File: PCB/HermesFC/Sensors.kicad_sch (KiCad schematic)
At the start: 16 parts, among them U4 MPU-6050, U5 BMP280, U6 LD39015M18R, U7 NTS0104PW, U8 ICM-20948

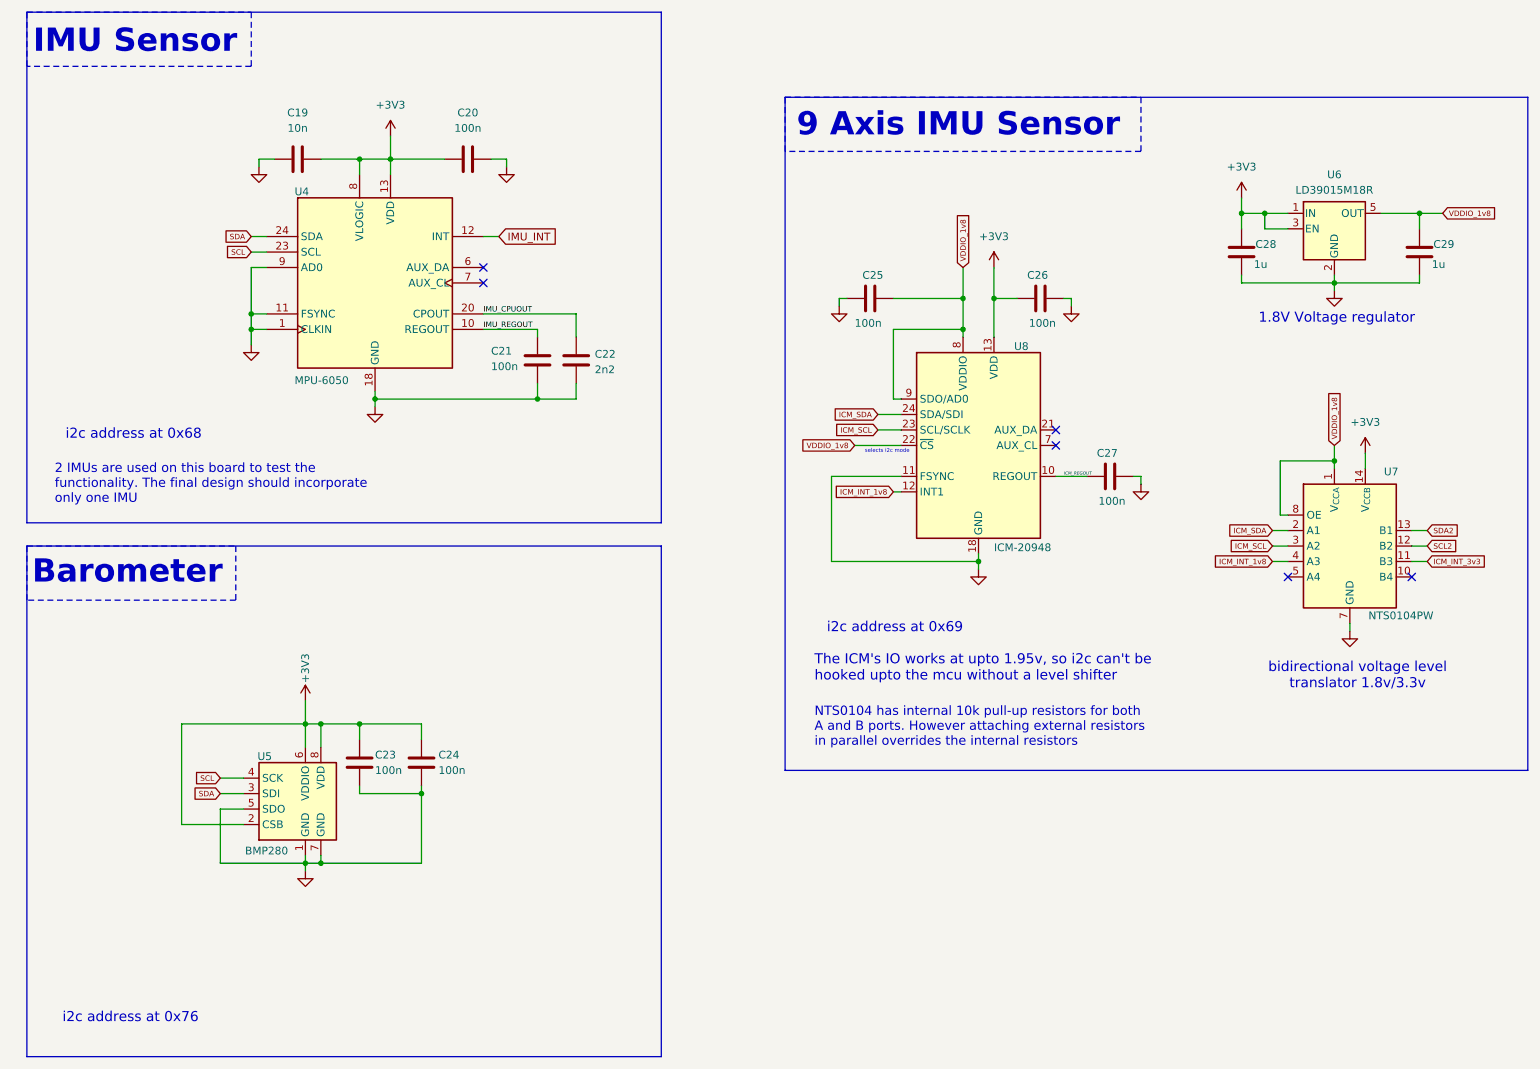
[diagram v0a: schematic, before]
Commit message: v0.2 updated schematic + PCB
added battery power source to PCB
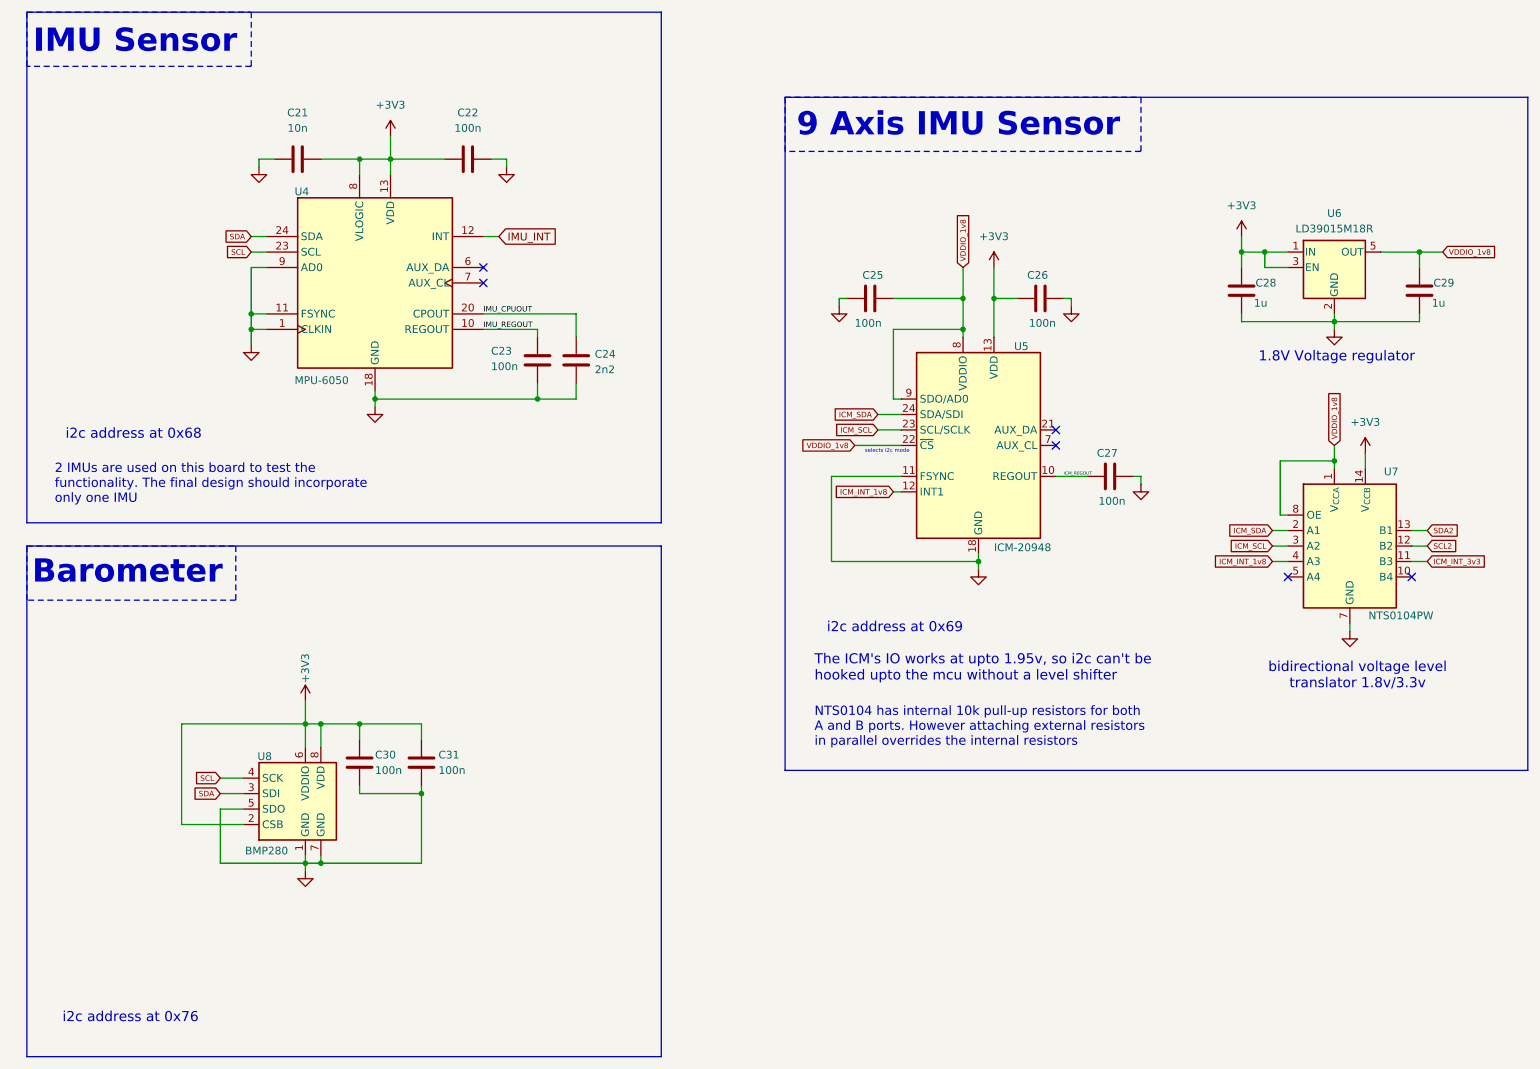
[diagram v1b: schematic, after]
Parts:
- C21: renamed from C19; footprint (none) -> Capacitor_SMD:C_0402_1005Metric
- C22: renamed from C20; footprint (none) -> Capacitor_SMD:C_0402_1005Metric
- C23: renamed from C21; footprint (none) -> Capacitor_SMD:C_0402_1005Metric
- C24: renamed from C22; footprint (none) -> Capacitor_SMD:C_0402_1005Metric
- C25, C26, C27, C28, C29: footprint (none) -> Capacitor_SMD:C_0402_1005Metric
- C30: renamed from C23; footprint (none) -> Capacitor_SMD:C_0402_1005Metric
- C31: renamed from C24; footprint (none) -> Capacitor_SMD:C_0402_1005Metric
- U7: footprint (none) -> Package_SO:TSSOP-14_4.4x5mm_P0.65mm
- renumbered U8 to U5, U5 to U8
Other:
- moved on the sheet: C28, C29, U6

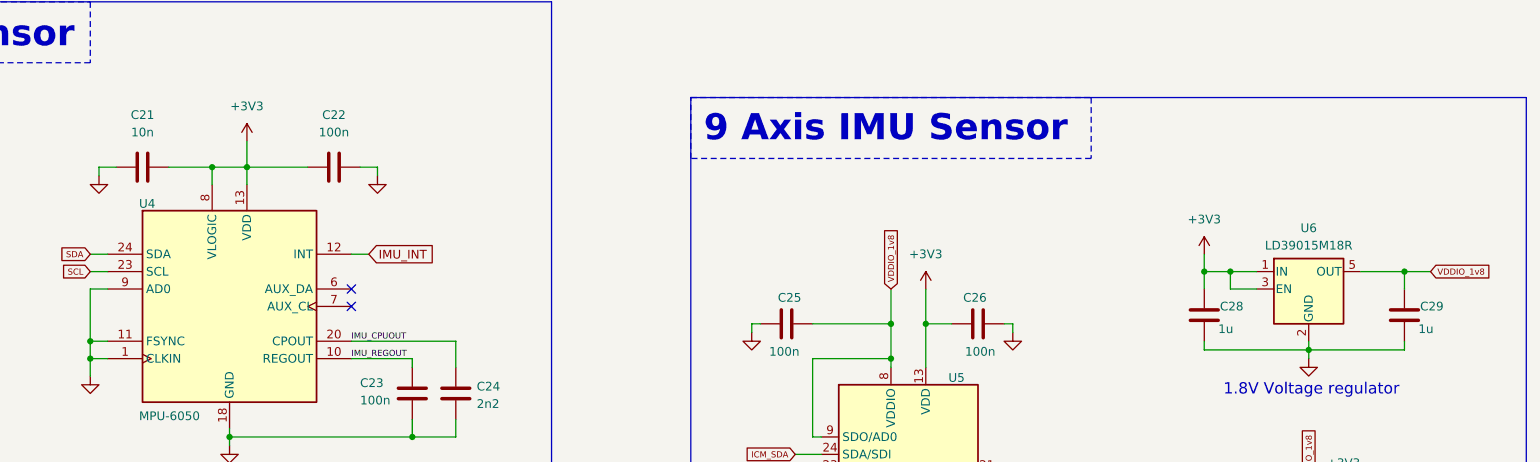
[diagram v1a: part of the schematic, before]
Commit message: Updated design files for optimized BOM
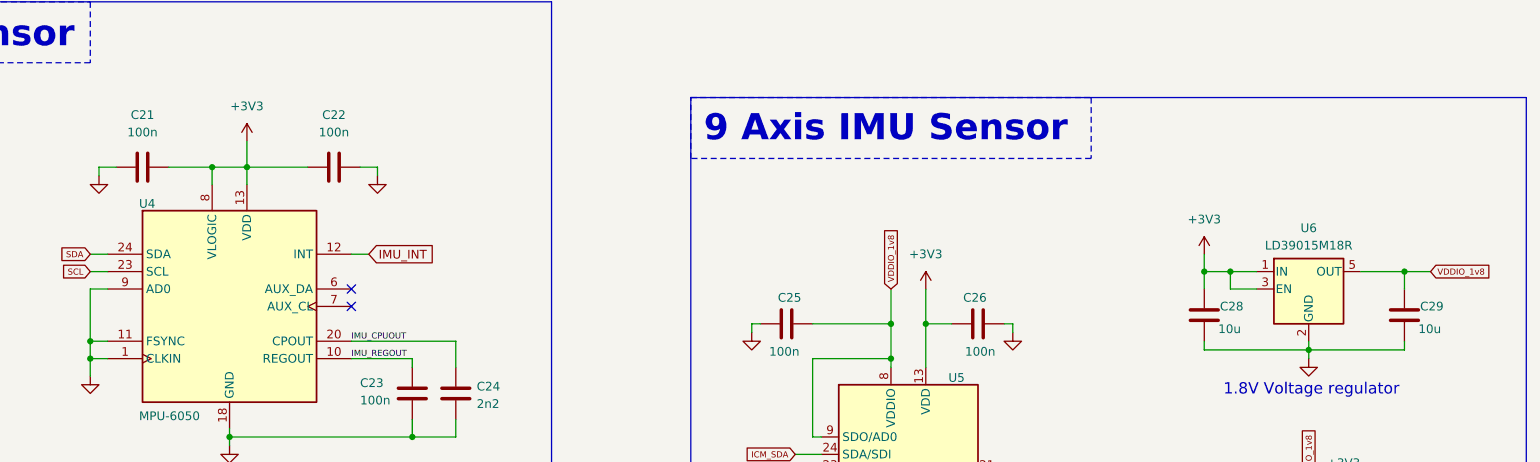
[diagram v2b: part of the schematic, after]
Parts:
- C21: value 10n -> 100n
- C24: footprint Capacitor_SMD:C_0402_1005Metric -> Capacitor_SMD:C_0603_1608Metric
- C28, C29: value 1u -> 10u; footprint Capacitor_SMD:C_0402_1005Metric -> Capacitor_SMD:C_0603_1608Metric
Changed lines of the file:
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@@
 			)
 		)
-		(property "Footprint" "Capacitor_SMD:C_0402_1005Metric"
+		(property "Footprint" "Capacitor_SMD:C_0603_1608Metric"
 			(at 116.5352 80.01 0)
 			(effects
@@
 			)
 		)
-		(property "Value" "10n"
+		(property "Value" "100n"
 			(at 69.85 38.1 90)
 			(effects
@@
 			)
 		)
-		(property "Value" "1u"
+		(property "Value" "10u"
 			(at 226.822 66.802 0)
 			(effects
@@
 			)
 		)
-		(property "Footprint" "Capacitor_SMD:C_0402_1005Metric"
+		(property "Footprint" "Capacitor_SMD:C_0603_1608Metric"
 			(at 225.7552 68.58 0)
 			(effects
@@
 			)
 		)
-		(property "Value" "1u"
+		(property "Value" "10u"
 			(at 256.032 66.802 0)
 			(effects
@@
 			)
 		)
-		(property "Footprint" "Capacitor_SMD:C_0402_1005Metric"
+		(property "Footprint" "Capacitor_SMD:C_0603_1608Metric"
 			(at 254.9652 68.58 0)
 			(effects
